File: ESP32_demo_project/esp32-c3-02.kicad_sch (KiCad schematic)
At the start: 15 parts, among them J3 GSD090012SEU, U3 ESP32-C3-WROOM-02-H4, U4 CP2102N-Axx-xQFN20, U5 USBLC6-2SC6, U6 W25Q32JVSSIQ

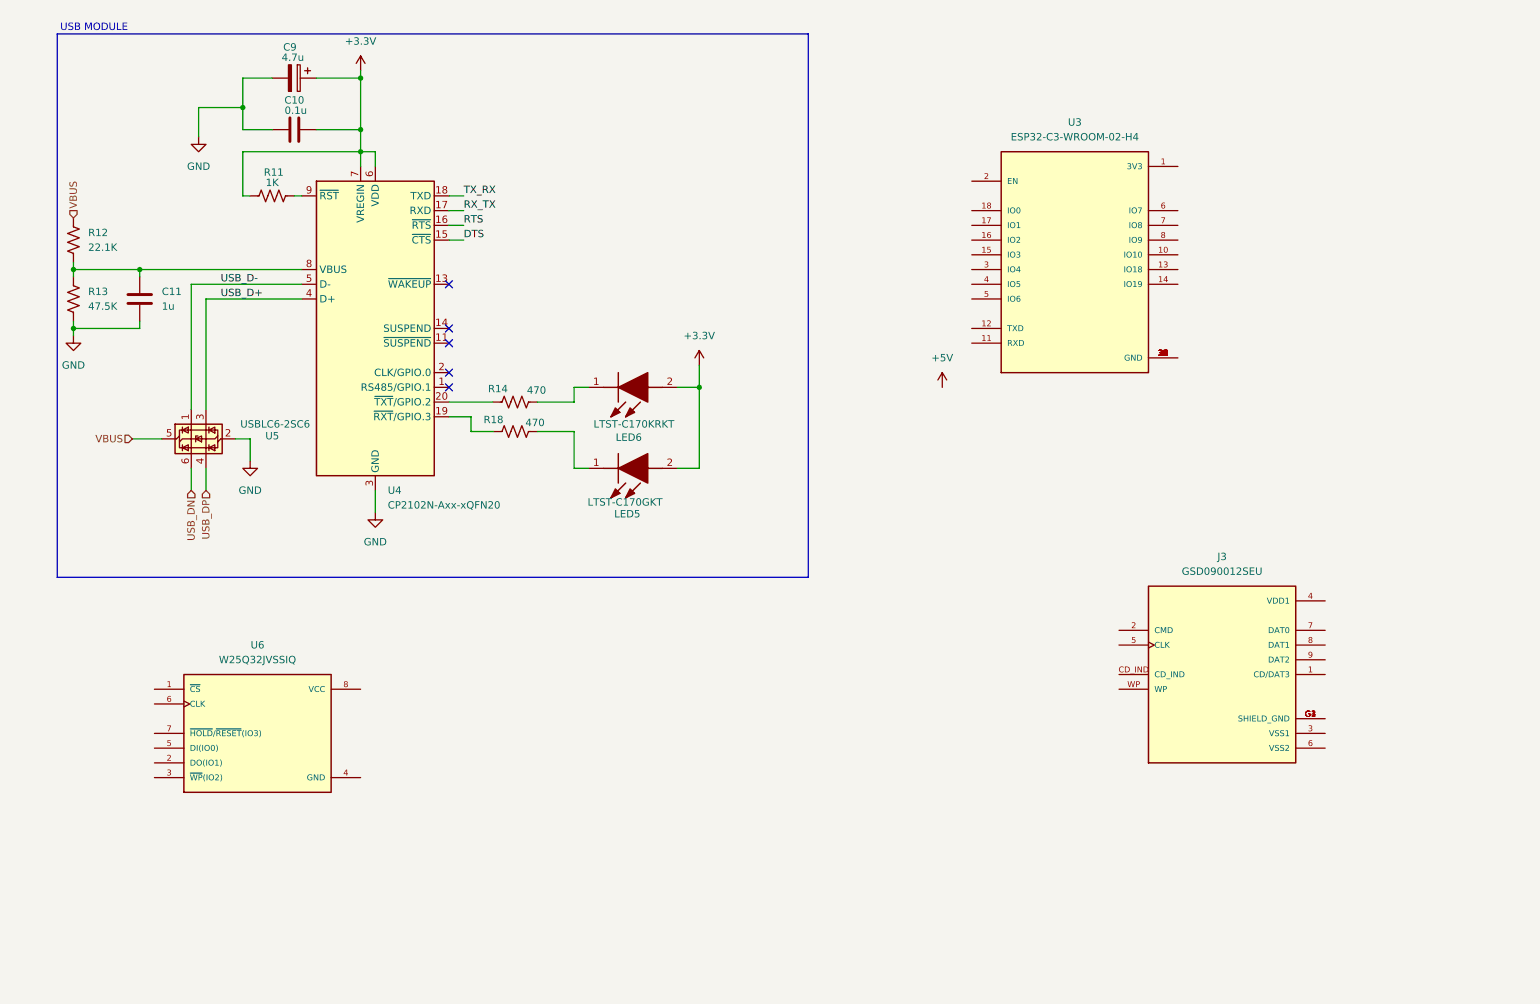
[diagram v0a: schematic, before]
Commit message: main: update to project
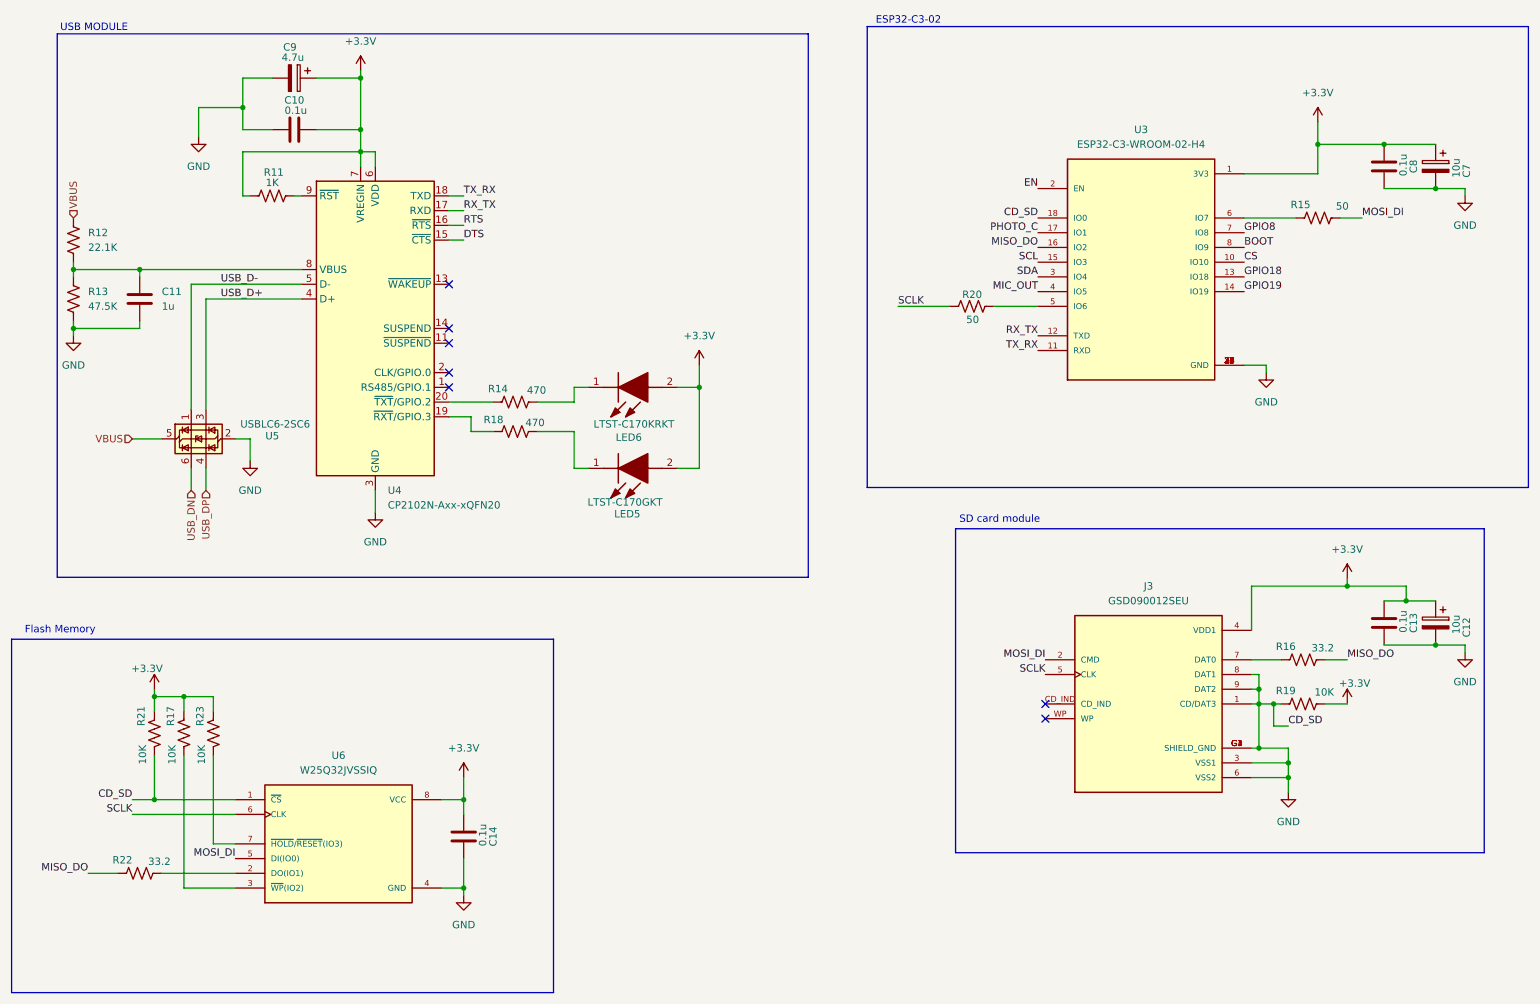
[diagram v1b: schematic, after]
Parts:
- added C12, C7: 10u, symbol Device:C_Polarized
- added C13, C14, C8: 0.1u, symbol Device:C
- added R15, R20: 50, symbol Device:R_US
- added R16, R22: 33.2, symbol Device:R_US
- added R17, R19, R21, R23: 10K, symbol Device:R_US
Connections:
- net +3.3V: now also J3.4 (VDD1), U3.1 (3V3), U6.8 (VCC), C12.1, C13.2, C14.2, C7.1, C8.2, R17.1, R19.2, R21.1, R23.1
- net GND: now also J3.1 (CD/DAT3), J3.3 (VSS1), J3.6 (VSS2), J3.8 (DAT1), J3.9 (DAT2), J3.G1 (SHIELD_GND), J3.G2 (SHIELD_GND), J3.G3 (SHIELD_GND), J3.G4 (SHIELD_GND), U3.18 (IO0), U3.19 (GND), U3.20 (GND), U3.21 (GND), U3.22 (GND), U3.23 (GND), U3.24 (GND), U3.25 (GND), U3.26 (GND), U3.27 (GND), U3.28 (GND), U3.29 (GND), U3.30 (GND), U3.31 (GND), U3.32 (GND), U3.33 (GND), U3.34 (GND), U3.35 (GND), U3.36 (GND), U3.37 (GND), U3.38 (GND), U3.39 (GND), U3.9 (GND), U6.1 (~{CS}), U6.4 (GND), C12.2, C13.1, C14.1, C7.2, C8.1, R19.1, R21.2
- net RX_TX: now also U3.12 (TXD)
- net TX_RX: now also U3.11 (RXD)
- net MOSI_DI: now reaches J3.2 (CMD)
- net MOSI_DI: now also U6.5 (DI(IO0)), R15.2
- net SCLK: now reaches J3.5 (CLK)
- net SCLK: now also U6.6 (CLK), R20.1
- net at J3.7 (DAT0): now also R16.1
- net at U6.2 (DO(IO1)): now also R22.2
- net at U6.3 (~{WP}(IO2)): now also R17.2
- net at U6.7 (~{HOLD}/~{RESET}(IO3)): now also R23.2
- net CS: now reaches U3.10 (IO10)
- net GPIO18: now reaches U3.13 (IO18)
- net GPIO19: now reaches U3.14 (IO19)
- net SCL: now reaches U3.15 (IO3)
- net MISO_DO: now reaches U3.16 (IO2)
- net MISO_DO: now also R16.2, R22.1
- net PHOTO_C: now reaches U3.17 (IO1)
- net EN: now reaches U3.2 (EN)
- net SDA: now reaches U3.3 (IO4)
- net MIC_OUT: now reaches U3.4 (IO5)
- net at U3.5 (IO6): now also R20.2
- net at U3.6 (IO7): now also R15.1
- net GPIO8: now reaches U3.7 (IO8)
- net BOOT: now reaches U3.8 (IO9)
- no-connect marks 5 -> 7
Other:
- note added: "ESP32-C3-02"
- note added: "Flash Memory"
- note added: "SD card module"
- moved on the sheet: J3, U3, U6
